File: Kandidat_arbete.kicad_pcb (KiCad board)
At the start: 4 copper layers, 100 x 75 mm, 97 parts, among them J100 Screw_Terminal_01x02, J2 USB_C_Receptacle_USB2.0, J200 Conn_02x05_Odd_Even, J201 Conn_01x04, J203 Conn_01x04, J204 Conn_01x04, J205 Conn_01x04, J207 Conn_01x05, J208 Conn_01x05, J209 Conn_01x05, J300 Conn_01x03, Q100 BSP 171, SW1 SW_Push, SW200 BOOT0, U1 LM5017MR, U101 LVR 3.3V, U200 STM32F405RGT6, U201 USBLC6-2SC6, Y200 16Mhz

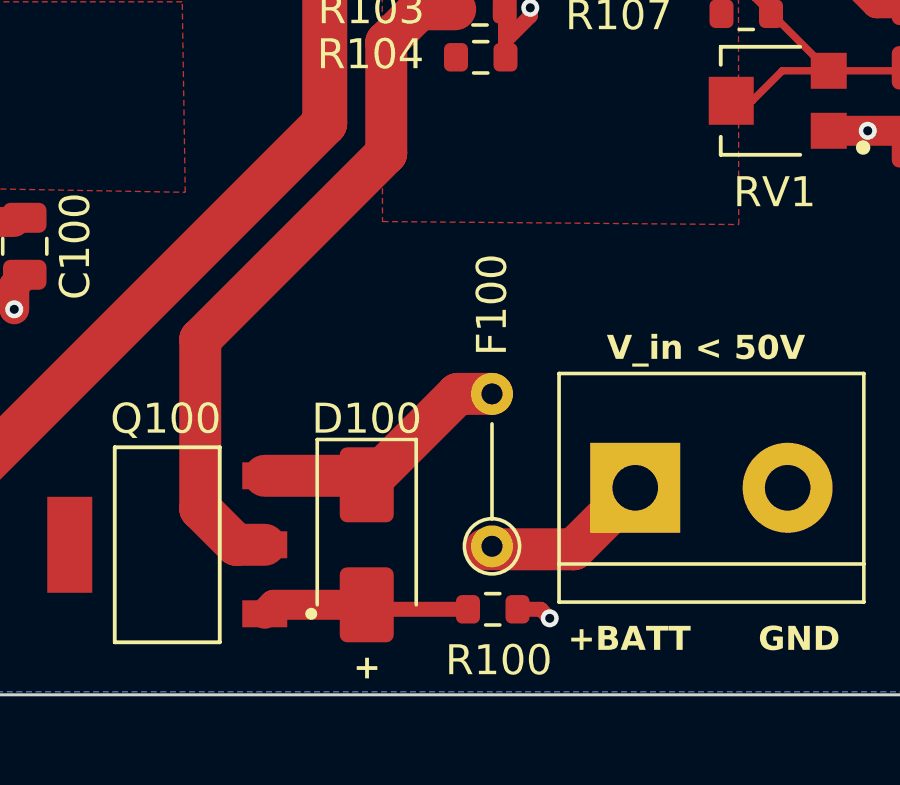
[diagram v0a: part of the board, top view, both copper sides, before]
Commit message: changes
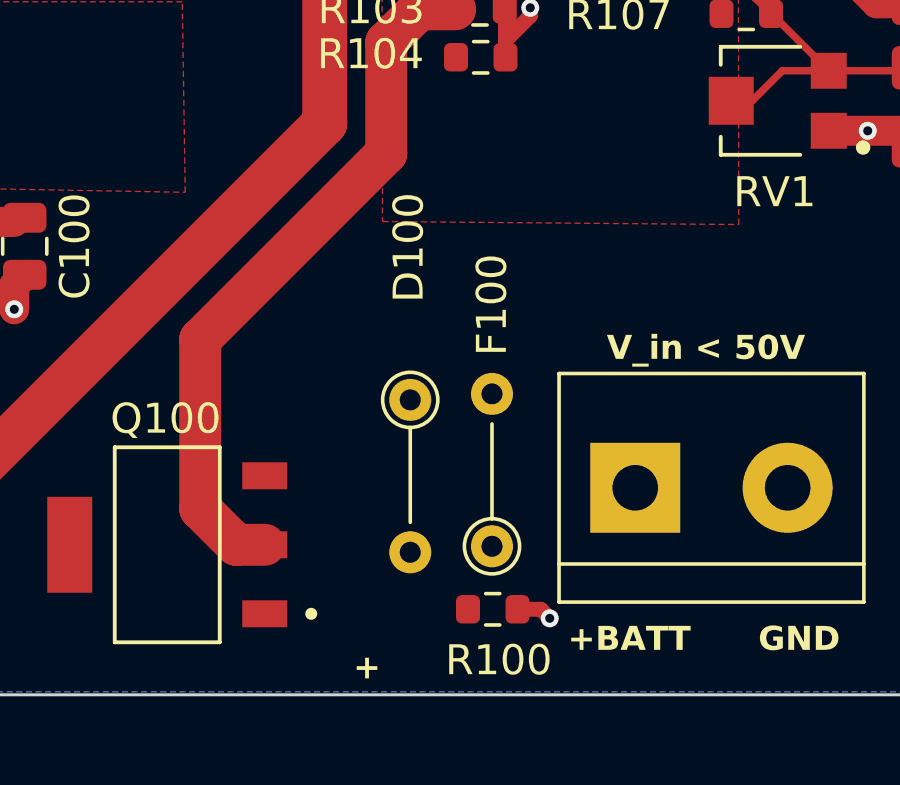
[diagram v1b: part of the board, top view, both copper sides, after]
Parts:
- D100: footprint Diode_SMD:D_SMA -> Resistor_THT:R_Axial_DIN0204_L3.6mm_D1.6mm_P5.08mm_Vertical
- moved D100 5.04 mm to (174.8, 140.2)
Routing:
- net Net-(D100-K): track 8.95 -> 0.00 mm
- net Net-(D100-A): track 6.96 -> 0.00 mm
- net +BATT: track 5.85 -> 0.00 mm
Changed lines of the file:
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@@
   (net 120 "unconnected-(HMC5883-15(DRDY)-Pad15)")
   (net 121 "unconnected-(U200-PC4-Pad24)")
-  (net 122 "Net-(U200-VCAP_1)")
-  (net 123 "Net-(U200-VCAP_2)")
+  (net 122 "Net-(#FLG0103-pwr)")
+  (net 123 "Net-(#FLG0104-pwr)")
   (net 124 "Net-(J2-CC1)")
   (net 125 "unconnected-(J2-SBU1-PadA8)")
@@
       (net 33 "I2C2_SDA") (pinfunction "PB11") (pintype "bidirectional"))
     (pad "31" smd roundrect (at 3.25 5.675) (size 0.3 1.55) (layers "F.Cu" "F.Paste" "F.Mask") (roundrect_rratio 0.25)
-      (net 122 "Net-(U200-VCAP_1)") (pinfunction "VCAP_1") (pintype "power_in"))
+      (net 122 "Net-(#FLG0103-pwr)") (pinfunction "VCAP_1") (pintype "power_in"))
     (pad "32" smd roundrect (at 3.75 5.675) (size 0.3 1.55) (layers "F.Cu" "F.Paste" "F.Mask") (roundrect_rratio 0.25)
       (net 2 "+3.3V") (pinfunction "VDD") (pintype "power_in"))
@@
       (net 57 "SWDIO") (pinfunction "PA13") (pintype "bidirectional"))
     (pad "47" smd roundrect (at 5.675 -3.25) (size 1.55 0.3) (layers "F.Cu" "F.Paste" "F.Mask") (roundrect_rratio 0.25)
-      (net 123 "Net-(U200-VCAP_2)") (pinfunction "VCAP_2") (pintype "power_in"))
+      (net 123 "Net-(#FLG0104-pwr)") (pinfunction "VCAP_2") (pintype "power_in"))
     (pad "48" smd roundrect (at 5.675 -3.75) (size 1.55 0.3) (layers "F.Cu" "F.Paste" "F.Mask") (roundrect_rratio 0.25)
       (net 2 "+3.3V") (pinfunction "VDD") (pintype "power_in"))
@@
       (stroke (width 0.1) (type solid)) (layer "F.Fab"))
     (pad "1" smd roundrect (at -0.775 0 270) (size 0.9 0.95) (layers "F.Cu" "F.Paste" "F.Mask") (roundrect_rratio 0.25)
-      (net 122 "Net-(U200-VCAP_1)") (pintype "passive"))
+      (net 122 "Net-(#FLG0103-pwr)") (pintype "passive"))
     (pad "2" smd roundrect (at 0.775 0 270) (size 0.9 0.95) (layers "F.Cu" "F.Paste" "F.Mask") (roundrect_rratio 0.25)
       (net 1 "GND") (pintype "passive"))
@@
       (stroke (width 0.1) (type solid)) (layer "F.Fab"))
     (pad "1" smd roundrect (at -0.775 0) (size 0.9 0.95) (layers "F.Cu" "F.Paste" "F.Mask") (roundrect_rratio 0.25)
-      (net 123 "Net-(U200-VCAP_2)") (pintype "passive"))
+      (net 123 "Net-(#FLG0104-pwr)") (pintype "passive"))
     (pad "2" smd roundrect (at 0.775 0) (size 0.9 0.95) (layers "F.Cu" "F.Paste" "F.Mask") (roundrect_rratio 0.25)
       (net 1 "GND") (pintype "passive"))
@@
     )
   )
-  (footprint "Diode_SMD:D_SMA" (layer "F.Cu")
-    (at 173.3 145 -90)
-    (descr "Diode SMA (DO-214AC)")
-    (tags "Diode SMA (DO-214AC)")
+  (footprint "Resistor_THT:R_Axial_DIN0204_L3.6mm_D1.6mm_P5.08mm_Vertical" (layer "F.Cu")
+    (at 174.75 140.17 -90)
+    (descr "Resistor, Axial_DIN0204 series, Axial, Vertical, pin pitch=5.08mm, 0.167W, length*diameter=3.6*1.6mm^2, http://cdn-reichelt.de/documents/datenblatt/B400/1_4W%23YAG.pdf")
+    (tags "Resistor Axial_DIN0204 series Axial Vertical pin pitch 5.08mm 0.167W length 3.6mm diameter 1.6mm")
     (property "Mouser" "")
     (property "PARTREV" "C8062")
@@
     (property "ki_description" "Zener diode, small symbol")
     (property "ki_keywords" "diode")
-    (attr smd)
-    (fp_text reference "D100" (at -4.2 0 -180) (layer "F.SilkS")
+    (attr through_hole)
+    (fp_text reference "D100" (at -5.08 0.05 -90) (layer "F.SilkS")
         (effects (font (size 1 1) (thickness 0.15)))
     )
-    (fp_text value "D_Zener_Small" (at 0 2.6 90) (layer "F.Fab")
+    (fp_text value "D_Zener_Small" (at 2.54 1.92 -90) (layer "F.Fab")
         (effects (font (size 1 1) (thickness 0.15)))
     )
-    (fp_text user "${REFERENCE}" (at 0 -2.5 90) (layer "F.Fab")
+    (fp_text user "${REFERENCE}" (at 2.54 -1.92 -90) (layer "F.Fab")
         (effects (font (size 1 1) (thickness 0.15)))
     )
-    (fp_line (start -3.51 -1.65) (end -3.51 1.65)
-      (stroke (width 0.12) (type solid)) (layer "F.SilkS"))
-    (fp_line (start -3.51 -1.65) (end 2 -1.65)
-      (stroke (width 0.12) (type solid)) (layer "F.SilkS"))
-    (fp_line (start -3.51 1.65) (end 2 1.65)
+    (fp_line (start 0.92 0) (end 4.08 0)
       (stroke (width 0.12) (type solid)) (layer "F.SilkS"))
-    (fp_line (start -3.5 -1.75) (end 3.5 -1.75)
+    (fp_circle (center 0 0) (end 0.92 0)
+      (stroke (width 0.12) (type solid)) (fill none) (layer "F.SilkS"))
+    (fp_line (start -1.05 -1.05) (end -1.05 1.05)
       (stroke (width 0.05) (type solid)) (layer "F.CrtYd"))
-    (fp_line (start -3.5 1.75) (end -3.5 -1.75)
+    (fp_line (start -1.05 1.05) (end 6.03 1.05)
       (stroke (width 0.05) (type solid)) (layer "F.CrtYd"))
-    (fp_line (start 3.5 -1.75) (end 3.5 1.75)
+    (fp_line (start 6.03 -1.05) (end -1.05 -1.05)
       (stroke (width 0.05) (type solid)) (layer "F.CrtYd"))
-    (fp_line (start 3.5 1.75) (end -3.5 1.75)
+    (fp_line (start 6.03 1.05) (end 6.03 -1.05)
       (stroke (width 0.05) (type solid)) (layer "F.CrtYd"))
-    (fp_line (start -2.3 1.5) (end -2.3 -1.5)
-      (stroke (width 0.1) (type solid)) (layer "F.Fab"))
-    (fp_line (start -0.64944 -0.79908) (end -0.64944 0.80112)
-      (stroke (width 0.1) (type solid)) (layer "F.Fab"))
-    (fp_line (start -0.64944 0.00102) (end -1.55114 0.00102)
-      (stroke (width 0.1) (type solid)) (layer "F.Fab"))
-    (fp_line (start -0.64944 0.00102) (end 0.50118 -0.79908)
-      (stroke (width 0.1) (type solid)) (layer "F.Fab"))
-    (fp_line (start -0.64944 0.00102) (end 0.50118 0.75032)
-      (stroke (width 0.1) (type solid)) (layer "F.Fab"))
-    (fp_line (start 0.50118 0.00102) (end 1.4994 0.00102)
-      (stroke (width 0.1) (type solid)) (layer "F.Fab"))
-    (fp_line (start 0.50118 0.75032) (end 0.50118 -0.79908)
-      (stroke (width 0.1) (type solid)) (layer "F.Fab"))
-    (fp_line (start 2.3 -1.5) (end -2.3 -1.5)
-      (stroke (width 0.1) (type solid)) (layer "F.Fab"))
-    (fp_line (start 2.3 -1.5) (end 2.3 1.5)
-      (stroke (width 0.1) (type solid)) (layer "F.Fab"))
-    (fp_line (start 2.3 1.5) (end -2.3 1.5)
+    (fp_line (start 0 0) (end 5.08 0)
       (stroke (width 0.1) (type solid)) (layer "F.Fab"))
-    (pad "1" smd roundrect (at -2 0 270) (size 2.5 1.8) (layers "F.Cu" "F.Paste" "F.Mask") (roundrect_rratio 0.1388888889)
+    (fp_circle (center 0 0) (end 0.8 0)
+      (stroke (width 0.1) (type solid)) (fill none) (layer "F.Fab"))
+    (pad "1" thru_hole circle (at 0 0 270) (size 1.4 1.4) (drill 0.7) (layers "*.Cu" "*.Mask")
       (net 16 "Net-(D100-K)") (pinfunction "K") (pintype "passive"))
-    (pad "2" smd roundrect (at 2 0 270) (size 2.5 1.8) (layers "F.Cu" "F.Paste" "F.Mask") (roundrect_rratio 0.1388888889)
+    (pad "2" thru_hole oval (at 5.08 0 270) (size 1.4 1.4) (drill 0.7) (layers "*.Cu" "*.Mask")
       (net 17 "Net-(D100-A)") (pinfunction "A") (pintype "passive"))
-    (model "${KICAD6_3DMODEL_DIR}/Diode_SMD.3dshapes/D_SMA.wrl"
+    (model "${KICAD6_3DMODEL_DIR}/Resistor_THT.3dshapes/R_Axial_DIN0204_L3.6mm_D1.6mm_P5.08mm_Vertical.wrl"
       (offset (xyz 0 0 0))
       (scale (xyz 1 1 1))
@@
   (segment (start 113.45 84.85) (end 112.87 85.43) (width 0.25) (layer "F.Cu") (net 15))
   (segment (start 112.87 85.43) (end 112.87 86.05) (width 0.25) (layer "F.Cu") (net 15))
-  (segment (start 169.9 142.7) (end 173 142.7) (width 1.4) (layer "F.Cu") (net 16))
-  (segment (start 176.33 139.97) (end 173.3 143) (width 1.4) (layer "F.Cu") (net 16))
-  (segment (start 173 142.7) (end 173.3 143) (width 1.4) (layer "F.Cu") (net 16))
-  (segment (start 177.475 139.97) (end 176.33 139.97) (width 1.4) (layer "F.Cu") (net 16))
-  (segment (start 173.45 147.15) (end 173.3 147) (width 0.25) (layer "F.Cu") (net 17))
-  (segment (start 170.2 147) (end 169.9 147.3) (width 1) (layer "F.Cu") (net 17))
-  (segment (start 173.3 147) (end 170.2 147) (width 1) (layer "F.Cu") (net 17))
-  (segment (start 176.675 147.15) (end 173.45 147.15) (width 0.5) (layer "F.Cu") (net 17))
   (segment (start 155.1 140.8) (end 156.8875 140.8) (width 0.25) (layer "F.Cu") (net 18))
   (segment (start 156.8875 140.8) (end 157 140.6875) (width 0.25) (layer "F.Cu") (net 18))
@@
   (segment (start 137.5 107.45) (end 137.2 107.15) (width 0.25) (layer "In2.Cu") (net 22))
   (segment (start 137.2 107.15) (end 120.85 107.15) (width 0.25) (layer "In2.Cu") (net 22))
-  (segment (start 177.25 145.15) (end 180.2 145.15) (width 1.4) (layer "F.Cu") (net 23))
-  (segment (start 180.2 145.15) (end 182.25 143.1) (width 1.4) (layer "F.Cu") (net 23))
   (segment (start 180.8875 109.875) (end 180.8875 111.6625) (width 0.25) (layer "F.Cu") (net 24))
   (segment (start 180.8875 111.6625) (end 181.2 111.975) (width 0.25) (layer "F.Cu") (net 24))

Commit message: Revert "changes"
This reverts commit 655f2439946f26e228e6387e4a45df3a138819d6.
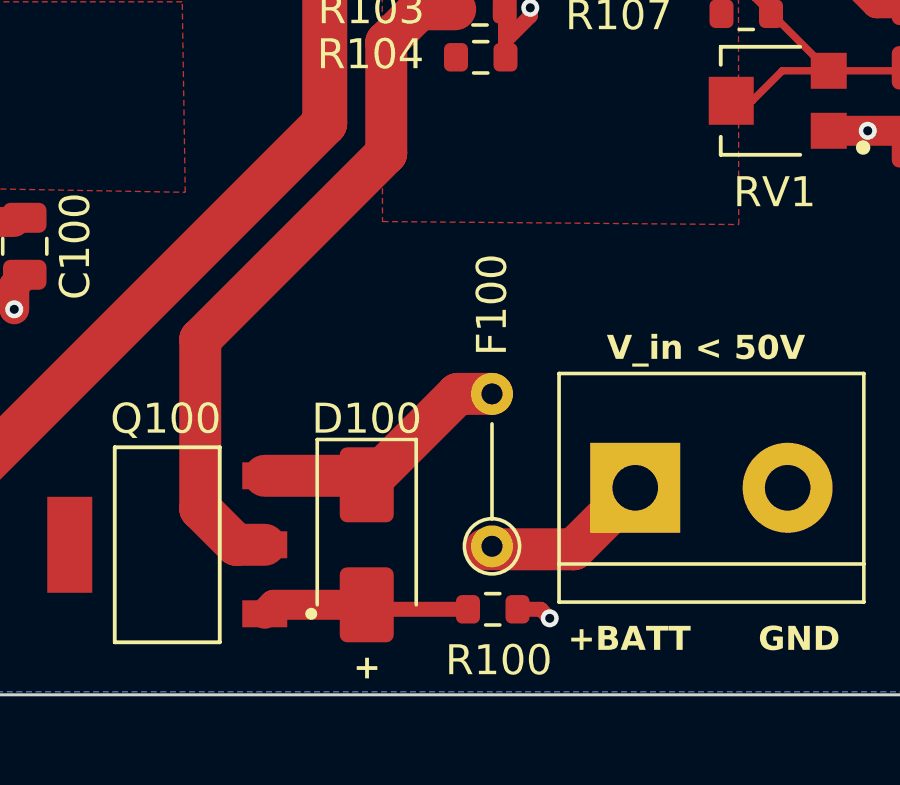
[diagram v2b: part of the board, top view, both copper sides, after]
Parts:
- D100: footprint Resistor_THT:R_Axial_DIN0204_L3.6mm_D1.6mm_P5.08mm_Vertical -> Diode_SMD:D_SMA
- moved D100 5.04 mm to (173.3, 145.0)
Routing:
- net Net-(D100-K): track 0.00 -> 8.95 mm
- net Net-(D100-A): track 0.00 -> 6.96 mm
- net +BATT: track 0.00 -> 5.85 mm
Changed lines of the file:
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@@
   (net 120 "unconnected-(HMC5883-15(DRDY)-Pad15)")
   (net 121 "unconnected-(U200-PC4-Pad24)")
-  (net 122 "Net-(#FLG0103-pwr)")
-  (net 123 "Net-(#FLG0104-pwr)")
+  (net 122 "Net-(U200-VCAP_1)")
+  (net 123 "Net-(U200-VCAP_2)")
   (net 124 "Net-(J2-CC1)")
   (net 125 "unconnected-(J2-SBU1-PadA8)")
@@
       (net 33 "I2C2_SDA") (pinfunction "PB11") (pintype "bidirectional"))
     (pad "31" smd roundrect (at 3.25 5.675) (size 0.3 1.55) (layers "F.Cu" "F.Paste" "F.Mask") (roundrect_rratio 0.25)
-      (net 122 "Net-(#FLG0103-pwr)") (pinfunction "VCAP_1") (pintype "power_in"))
+      (net 122 "Net-(U200-VCAP_1)") (pinfunction "VCAP_1") (pintype "power_in"))
     (pad "32" smd roundrect (at 3.75 5.675) (size 0.3 1.55) (layers "F.Cu" "F.Paste" "F.Mask") (roundrect_rratio 0.25)
       (net 2 "+3.3V") (pinfunction "VDD") (pintype "power_in"))
@@
       (net 57 "SWDIO") (pinfunction "PA13") (pintype "bidirectional"))
     (pad "47" smd roundrect (at 5.675 -3.25) (size 1.55 0.3) (layers "F.Cu" "F.Paste" "F.Mask") (roundrect_rratio 0.25)
-      (net 123 "Net-(#FLG0104-pwr)") (pinfunction "VCAP_2") (pintype "power_in"))
+      (net 123 "Net-(U200-VCAP_2)") (pinfunction "VCAP_2") (pintype "power_in"))
     (pad "48" smd roundrect (at 5.675 -3.75) (size 1.55 0.3) (layers "F.Cu" "F.Paste" "F.Mask") (roundrect_rratio 0.25)
       (net 2 "+3.3V") (pinfunction "VDD") (pintype "power_in"))
@@
       (stroke (width 0.1) (type solid)) (layer "F.Fab"))
     (pad "1" smd roundrect (at -0.775 0 270) (size 0.9 0.95) (layers "F.Cu" "F.Paste" "F.Mask") (roundrect_rratio 0.25)
-      (net 122 "Net-(#FLG0103-pwr)") (pintype "passive"))
+      (net 122 "Net-(U200-VCAP_1)") (pintype "passive"))
     (pad "2" smd roundrect (at 0.775 0 270) (size 0.9 0.95) (layers "F.Cu" "F.Paste" "F.Mask") (roundrect_rratio 0.25)
       (net 1 "GND") (pintype "passive"))
@@
       (stroke (width 0.1) (type solid)) (layer "F.Fab"))
     (pad "1" smd roundrect (at -0.775 0) (size 0.9 0.95) (layers "F.Cu" "F.Paste" "F.Mask") (roundrect_rratio 0.25)
-      (net 123 "Net-(#FLG0104-pwr)") (pintype "passive"))
+      (net 123 "Net-(U200-VCAP_2)") (pintype "passive"))
     (pad "2" smd roundrect (at 0.775 0) (size 0.9 0.95) (layers "F.Cu" "F.Paste" "F.Mask") (roundrect_rratio 0.25)
       (net 1 "GND") (pintype "passive"))
@@
     )
   )
-  (footprint "Resistor_THT:R_Axial_DIN0204_L3.6mm_D1.6mm_P5.08mm_Vertical" (layer "F.Cu")
-    (at 174.75 140.17 -90)
-    (descr "Resistor, Axial_DIN0204 series, Axial, Vertical, pin pitch=5.08mm, 0.167W, length*diameter=3.6*1.6mm^2, http://cdn-reichelt.de/documents/datenblatt/B400/1_4W%23YAG.pdf")
-    (tags "Resistor Axial_DIN0204 series Axial Vertical pin pitch 5.08mm 0.167W length 3.6mm diameter 1.6mm")
+  (footprint "Diode_SMD:D_SMA" (layer "F.Cu")
+    (at 173.3 145 -90)
+    (descr "Diode SMA (DO-214AC)")
+    (tags "Diode SMA (DO-214AC)")
     (property "Mouser" "")
     (property "PARTREV" "C8062")
@@
     (property "ki_description" "Zener diode, small symbol")
     (property "ki_keywords" "diode")
-    (attr through_hole)
-    (fp_text reference "D100" (at -5.08 0.05 -90) (layer "F.SilkS")
+    (attr smd)
+    (fp_text reference "D100" (at -4.2 0 -180) (layer "F.SilkS")
         (effects (font (size 1 1) (thickness 0.15)))
     )
-    (fp_text value "D_Zener_Small" (at 2.54 1.92 -90) (layer "F.Fab")
+    (fp_text value "D_Zener_Small" (at 0 2.6 90) (layer "F.Fab")
         (effects (font (size 1 1) (thickness 0.15)))
     )
-    (fp_text user "${REFERENCE}" (at 2.54 -1.92 -90) (layer "F.Fab")
+    (fp_text user "${REFERENCE}" (at 0 -2.5 90) (layer "F.Fab")
         (effects (font (size 1 1) (thickness 0.15)))
     )
-    (fp_line (start 0.92 0) (end 4.08 0)
+    (fp_line (start -3.51 -1.65) (end -3.51 1.65)
       (stroke (width 0.12) (type solid)) (layer "F.SilkS"))
-    (fp_circle (center 0 0) (end 0.92 0)
-      (stroke (width 0.12) (type solid)) (fill none) (layer "F.SilkS"))
-    (fp_line (start -1.05 -1.05) (end -1.05 1.05)
+    (fp_line (start -3.51 -1.65) (end 2 -1.65)
+      (stroke (width 0.12) (type solid)) (layer "F.SilkS"))
+    (fp_line (start -3.51 1.65) (end 2 1.65)
+      (stroke (width 0.12) (type solid)) (layer "F.SilkS"))
+    (fp_line (start -3.5 -1.75) (end 3.5 -1.75)
       (stroke (width 0.05) (type solid)) (layer "F.CrtYd"))
-    (fp_line (start -1.05 1.05) (end 6.03 1.05)
+    (fp_line (start -3.5 1.75) (end -3.5 -1.75)
       (stroke (width 0.05) (type solid)) (layer "F.CrtYd"))
-    (fp_line (start 6.03 -1.05) (end -1.05 -1.05)
+    (fp_line (start 3.5 -1.75) (end 3.5 1.75)
       (stroke (width 0.05) (type solid)) (layer "F.CrtYd"))
-    (fp_line (start 6.03 1.05) (end 6.03 -1.05)
+    (fp_line (start 3.5 1.75) (end -3.5 1.75)
       (stroke (width 0.05) (type solid)) (layer "F.CrtYd"))
-    (fp_line (start 0 0) (end 5.08 0)
+    (fp_line (start -2.3 1.5) (end -2.3 -1.5)
       (stroke (width 0.1) (type solid)) (layer "F.Fab"))
-    (fp_circle (center 0 0) (end 0.8 0)
-      (stroke (width 0.1) (type solid)) (fill none) (layer "F.Fab"))
-    (pad "1" thru_hole circle (at 0 0 270) (size 1.4 1.4) (drill 0.7) (layers "*.Cu" "*.Mask")
+    (fp_line (start -0.64944 -0.79908) (end -0.64944 0.80112)
+      (stroke (width 0.1) (type solid)) (layer "F.Fab"))
+    (fp_line (start -0.64944 0.00102) (end -1.55114 0.00102)
+      (stroke (width 0.1) (type solid)) (layer "F.Fab"))
+    (fp_line (start -0.64944 0.00102) (end 0.50118 -0.79908)
+      (stroke (width 0.1) (type solid)) (layer "F.Fab"))
+    (fp_line (start -0.64944 0.00102) (end 0.50118 0.75032)
+      (stroke (width 0.1) (type solid)) (layer "F.Fab"))
+    (fp_line (start 0.50118 0.00102) (end 1.4994 0.00102)
+      (stroke (width 0.1) (type solid)) (layer "F.Fab"))
+    (fp_line (start 0.50118 0.75032) (end 0.50118 -0.79908)
+      (stroke (width 0.1) (type solid)) (layer "F.Fab"))
+    (fp_line (start 2.3 -1.5) (end -2.3 -1.5)
+      (stroke (width 0.1) (type solid)) (layer "F.Fab"))
+    (fp_line (start 2.3 -1.5) (end 2.3 1.5)
+      (stroke (width 0.1) (type solid)) (layer "F.Fab"))
+    (fp_line (start 2.3 1.5) (end -2.3 1.5)
+      (stroke (width 0.1) (type solid)) (layer "F.Fab"))
+    (pad "1" smd roundrect (at -2 0 270) (size 2.5 1.8) (layers "F.Cu" "F.Paste" "F.Mask") (roundrect_rratio 0.1388888889)
       (net 16 "Net-(D100-K)") (pinfunction "K") (pintype "passive"))
-    (pad "2" thru_hole oval (at 5.08 0 270) (size 1.4 1.4) (drill 0.7) (layers "*.Cu" "*.Mask")
+    (pad "2" smd roundrect (at 2 0 270) (size 2.5 1.8) (layers "F.Cu" "F.Paste" "F.Mask") (roundrect_rratio 0.1388888889)
       (net 17 "Net-(D100-A)") (pinfunction "A") (pintype "passive"))
-    (model "${KICAD6_3DMODEL_DIR}/Resistor_THT.3dshapes/R_Axial_DIN0204_L3.6mm_D1.6mm_P5.08mm_Vertical.wrl"
+    (model "${KICAD6_3DMODEL_DIR}/Diode_SMD.3dshapes/D_SMA.wrl"
       (offset (xyz 0 0 0))
       (scale (xyz 1 1 1))
@@
   (segment (start 113.45 84.85) (end 112.87 85.43) (width 0.25) (layer "F.Cu") (net 15))
   (segment (start 112.87 85.43) (end 112.87 86.05) (width 0.25) (layer "F.Cu") (net 15))
+  (segment (start 169.9 142.7) (end 173 142.7) (width 1.4) (layer "F.Cu") (net 16))
+  (segment (start 176.33 139.97) (end 173.3 143) (width 1.4) (layer "F.Cu") (net 16))
+  (segment (start 173 142.7) (end 173.3 143) (width 1.4) (layer "F.Cu") (net 16))
+  (segment (start 177.475 139.97) (end 176.33 139.97) (width 1.4) (layer "F.Cu") (net 16))
+  (segment (start 173.45 147.15) (end 173.3 147) (width 0.25) (layer "F.Cu") (net 17))
+  (segment (start 170.2 147) (end 169.9 147.3) (width 1) (layer "F.Cu") (net 17))
+  (segment (start 173.3 147) (end 170.2 147) (width 1) (layer "F.Cu") (net 17))
+  (segment (start 176.675 147.15) (end 173.45 147.15) (width 0.5) (layer "F.Cu") (net 17))
   (segment (start 155.1 140.8) (end 156.8875 140.8) (width 0.25) (layer "F.Cu") (net 18))
   (segment (start 156.8875 140.8) (end 157 140.6875) (width 0.25) (layer "F.Cu") (net 18))
@@
   (segment (start 137.5 107.45) (end 137.2 107.15) (width 0.25) (layer "In2.Cu") (net 22))
   (segment (start 137.2 107.15) (end 120.85 107.15) (width 0.25) (layer "In2.Cu") (net 22))
+  (segment (start 177.25 145.15) (end 180.2 145.15) (width 1.4) (layer "F.Cu") (net 23))
+  (segment (start 180.2 145.15) (end 182.25 143.1) (width 1.4) (layer "F.Cu") (net 23))
   (segment (start 180.8875 109.875) (end 180.8875 111.6625) (width 0.25) (layer "F.Cu") (net 24))
   (segment (start 180.8875 111.6625) (end 181.2 111.975) (width 0.25) (layer "F.Cu") (net 24))
